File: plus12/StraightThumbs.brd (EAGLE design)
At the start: 118.7 x 54 mm, 14 parts

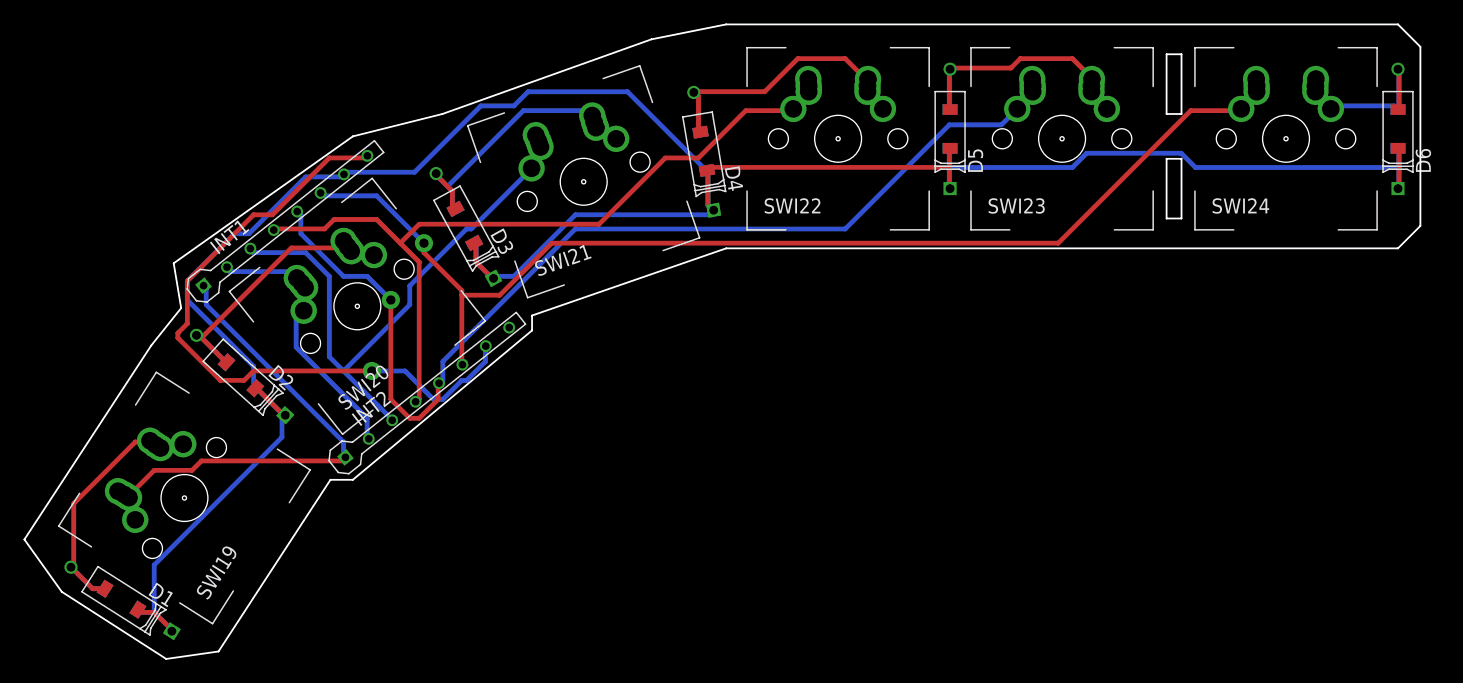
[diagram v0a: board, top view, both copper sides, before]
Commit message: Kobe beefing it up
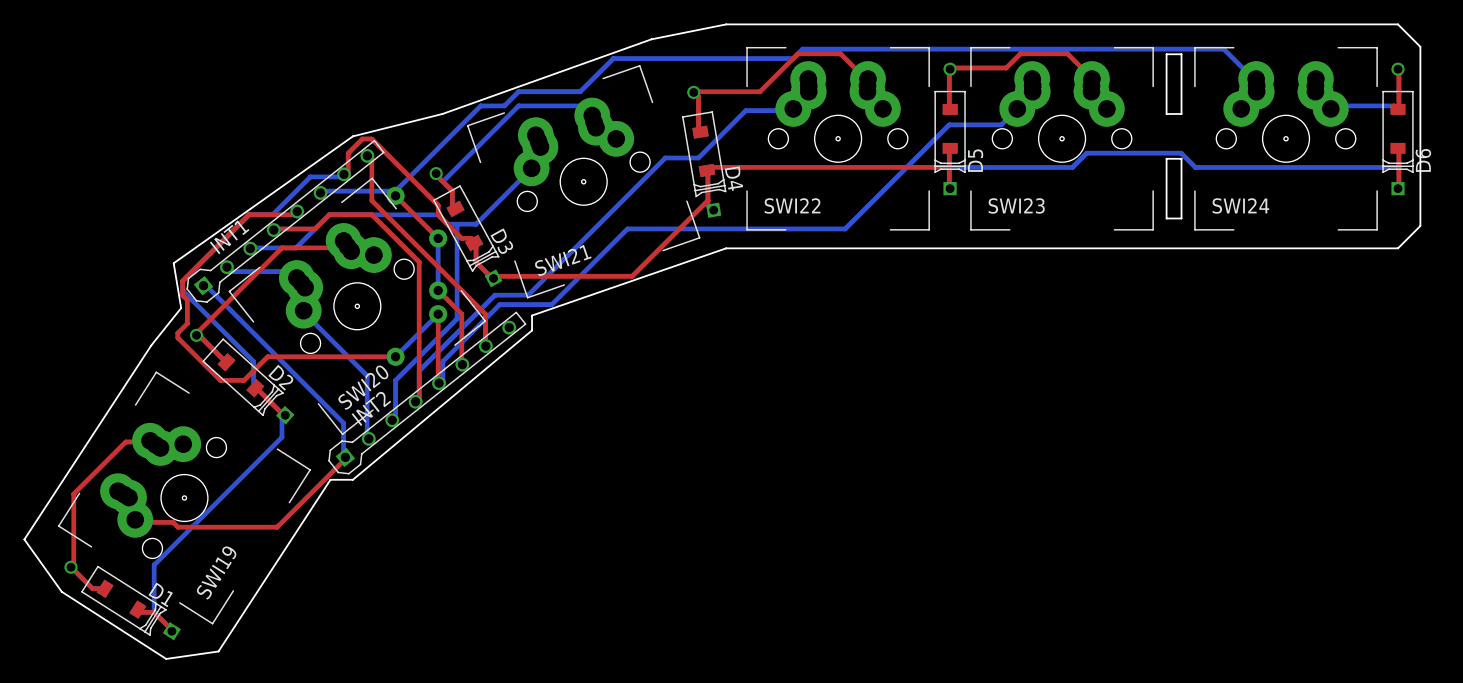
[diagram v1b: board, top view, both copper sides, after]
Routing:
- net N$14: track 56.6 -> 20.4 mm, vias 1 -> 0
- net N$11: track 90.9 -> 112.7 mm, vias 1 -> 2
- net N$13: track 211.1 -> 192.3 mm
- net N$12: track 99.5 -> 105.8 mm, vias 1 -> 3
- net N$10: track 68.8 -> 74.5 mm
- net N$5: track 20.6 -> 21.5 mm
- net N$8: track 24.7 -> 25.5 mm
- net N$3: track 22.4 -> 23.0 mm
- net N$7: track 44.0 -> 44.5 mm
